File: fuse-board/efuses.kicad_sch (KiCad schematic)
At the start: 63 parts, among them U10 TPS259830ONRGER, U11 TPS259830ONRGER, U12 TPS259830ONRGER, U4 TPS259830ONRGER, U5 TPS259830ONRGER, U6 TPS259830ONRGER, U7 TPS259830ONRGER, U8 TPS259830ONRGER, U9 TPS259830ONRGER

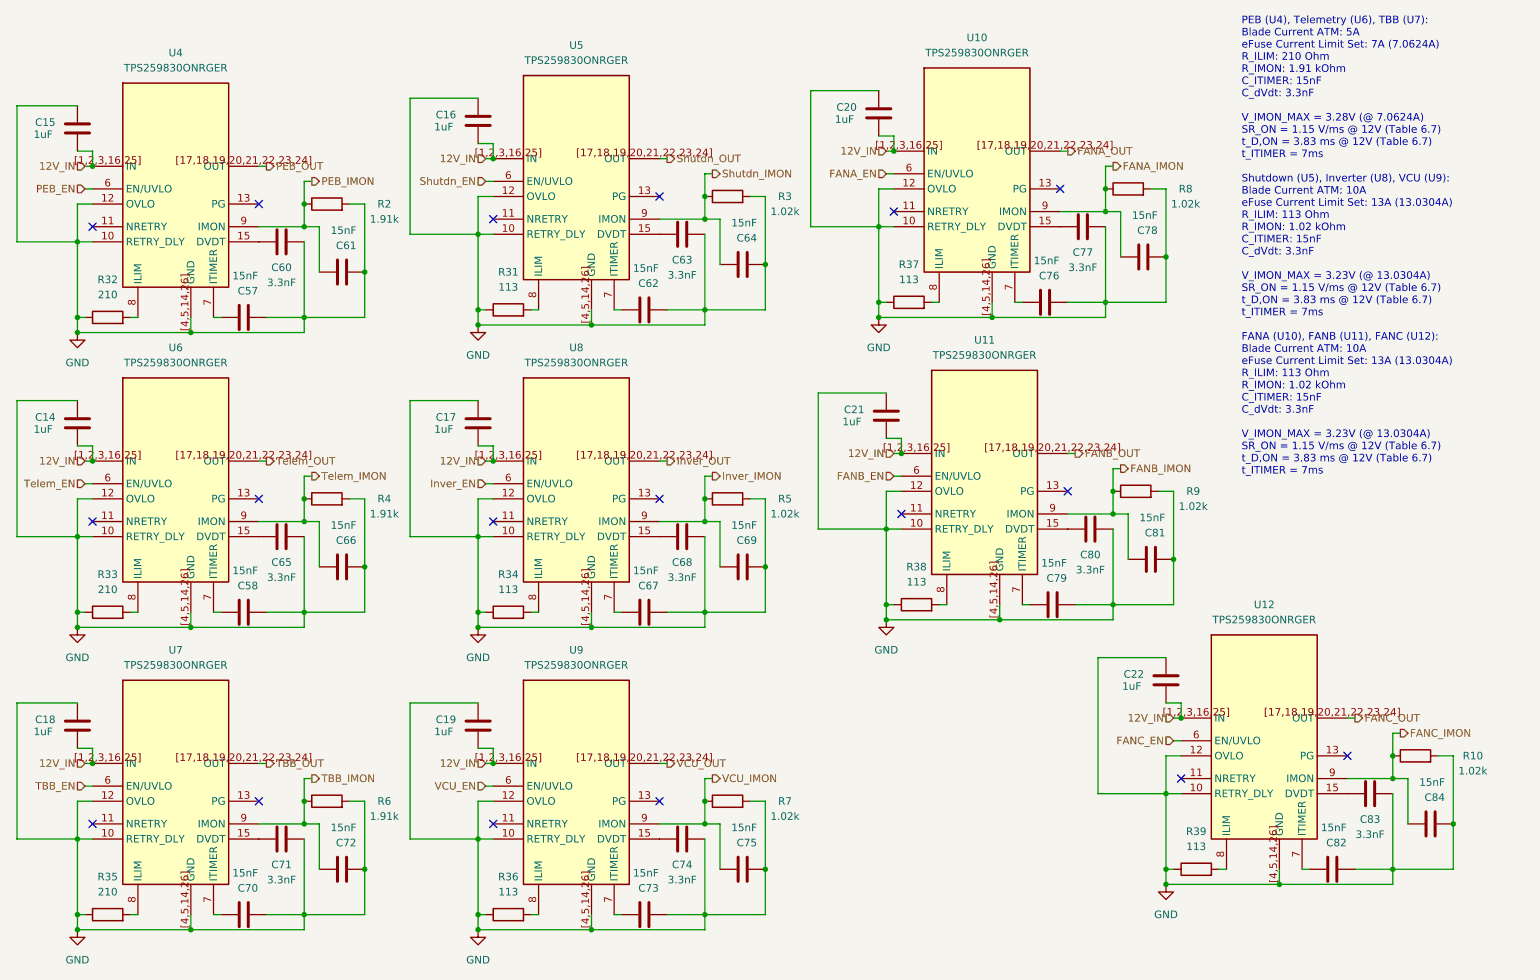
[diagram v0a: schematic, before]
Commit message: fix RC filters
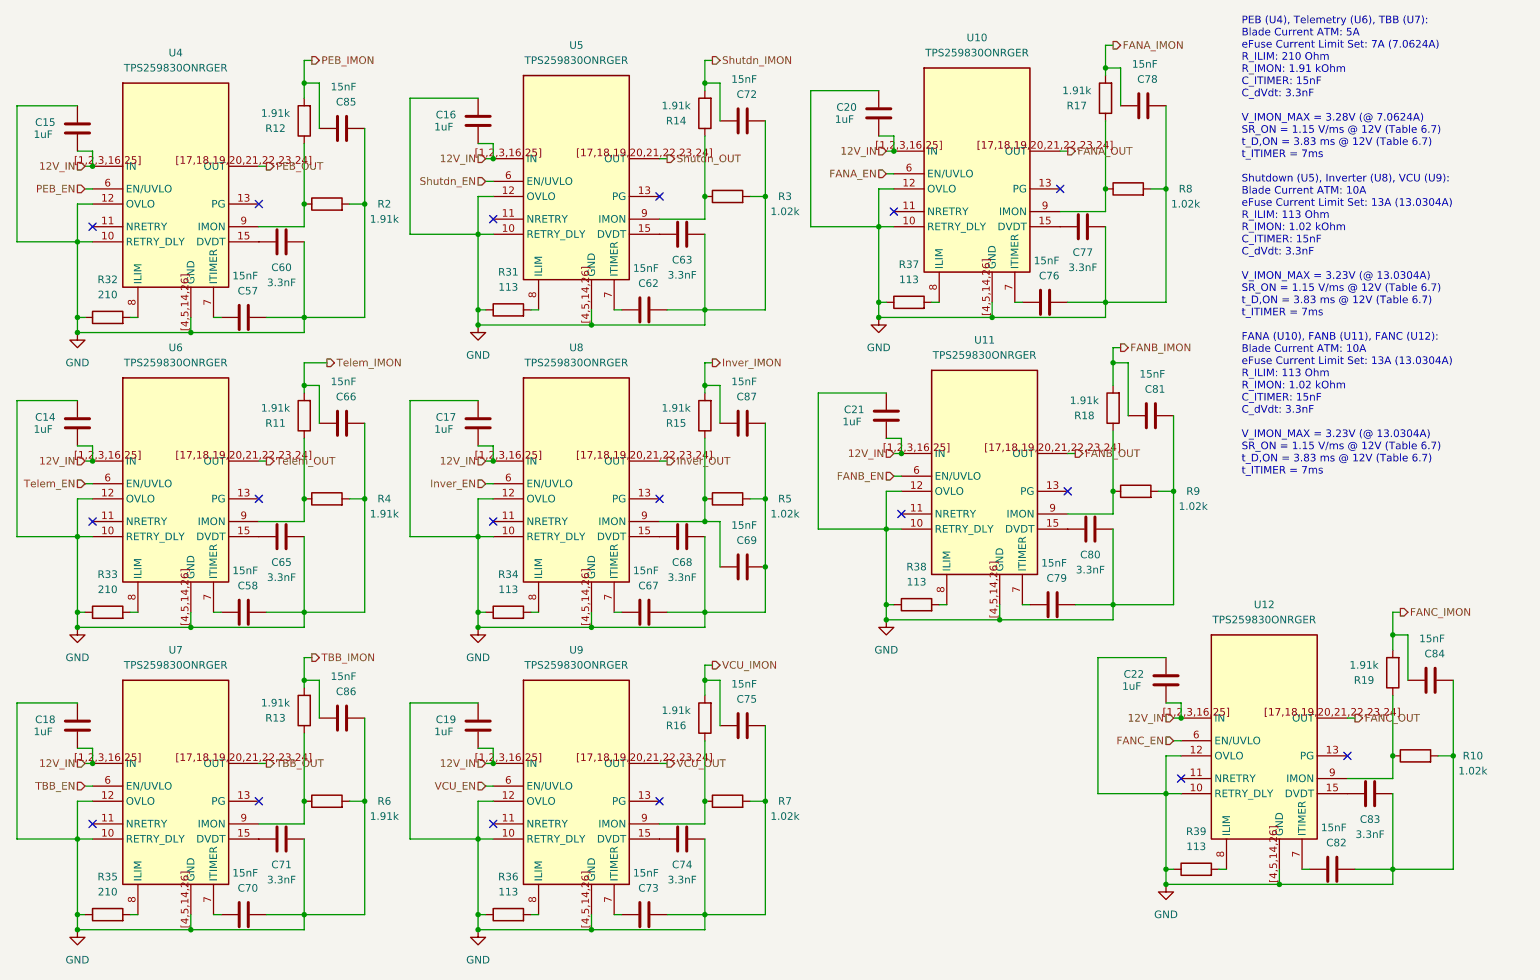
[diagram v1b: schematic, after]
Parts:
- removed C61, C64: 15nF, Capacitor_SMD:C_0603_1608Metric_Pad1.08x0.95mm_HandSolder, symbol Device:C
- added C85, C86, C87: 15nF, Capacitor_SMD:C_0603_1608Metric_Pad1.08x0.95mm_HandSolder, symbol Device:C
- added R11, R12, R13, R14, R15, R16, R17, R18, R19: 1.91k, Resistor_SMD:R_0603_1608Metric_Pad0.98x0.95mm_HandSolder, symbol Device:R
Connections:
- net FANA_IMON: now also R17.2; no longer R8.1, U10.9 (IMON)
- net FANB_IMON: now also R18.2; no longer R9.1, U11.9 (IMON)
- net FANC_IMON: now also R19.2; no longer R10.1, U12.9 (IMON)
- net GND: now also C85.2, C86.2, C87.2
- net Inver_IMON: now also C87.1, R15.2; no longer C69.1, R5.1, U8.9 (IMON)
- net PEB_IMON: now also C85.1, R12.2; no longer R2.1, U4.9 (IMON)
- net Shutdn_IMON: now also C72.1, R14.2; no longer R3.1, U5.9 (IMON)
- net TBB_IMON: now also C86.1, R13.2; no longer C72.1, R6.1, U7.9 (IMON)
- net Telem_IMON: now also R11.2; no longer R4.1, U6.9 (IMON)
- net VCU_IMON: now also R16.2; no longer R7.1, U9.9 (IMON)
- new net: C69.1, R15.1, R5.1, U8.9 (IMON)
- new net: R12.1, R2.1, U4.9 (IMON)
- new net: R11.1, R4.1, U6.9 (IMON)
- new net: R14.1, R3.1, U5.9 (IMON)
- new net: R16.1, R7.1, U9.9 (IMON)
- new net: R13.1, R6.1, U7.9 (IMON)
- new net: R18.1, R9.1, U11.9 (IMON)
- new net: R17.1, R8.1, U10.9 (IMON)
- new net: R10.1, R19.1, U12.9 (IMON)
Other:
- moved on the sheet: C66
